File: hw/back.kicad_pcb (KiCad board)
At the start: 2 copper layers, 110 x 55 mm, 77 parts, among them J1 IDC_02X13, J2 FC681495, J3 N42GK-04, Q1 BSC080N03MS, U1 OSRB38C9BA, U2 MCP1826S, U3 MCP1826S, U4 BQ24192, U5 LTC1871, U6 LTC2941CMS8E

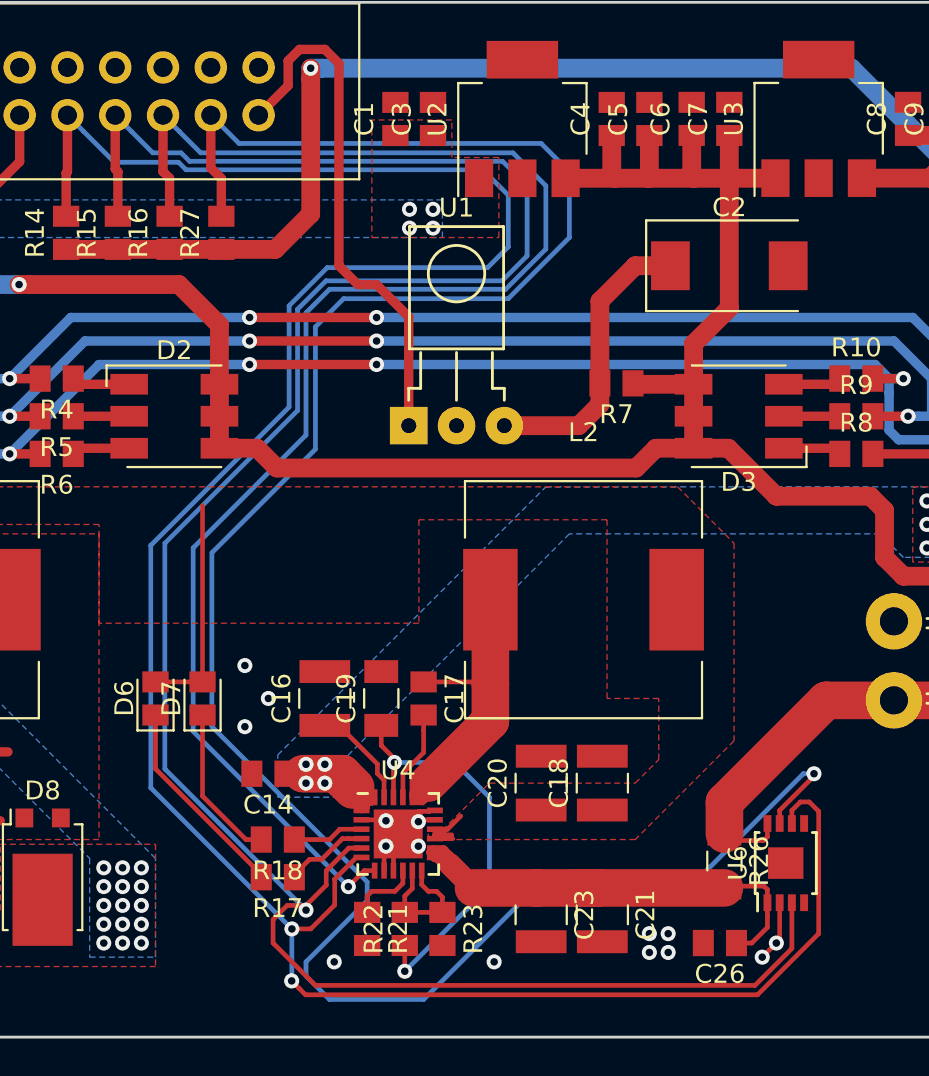
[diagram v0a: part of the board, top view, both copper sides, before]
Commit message: updated pcb
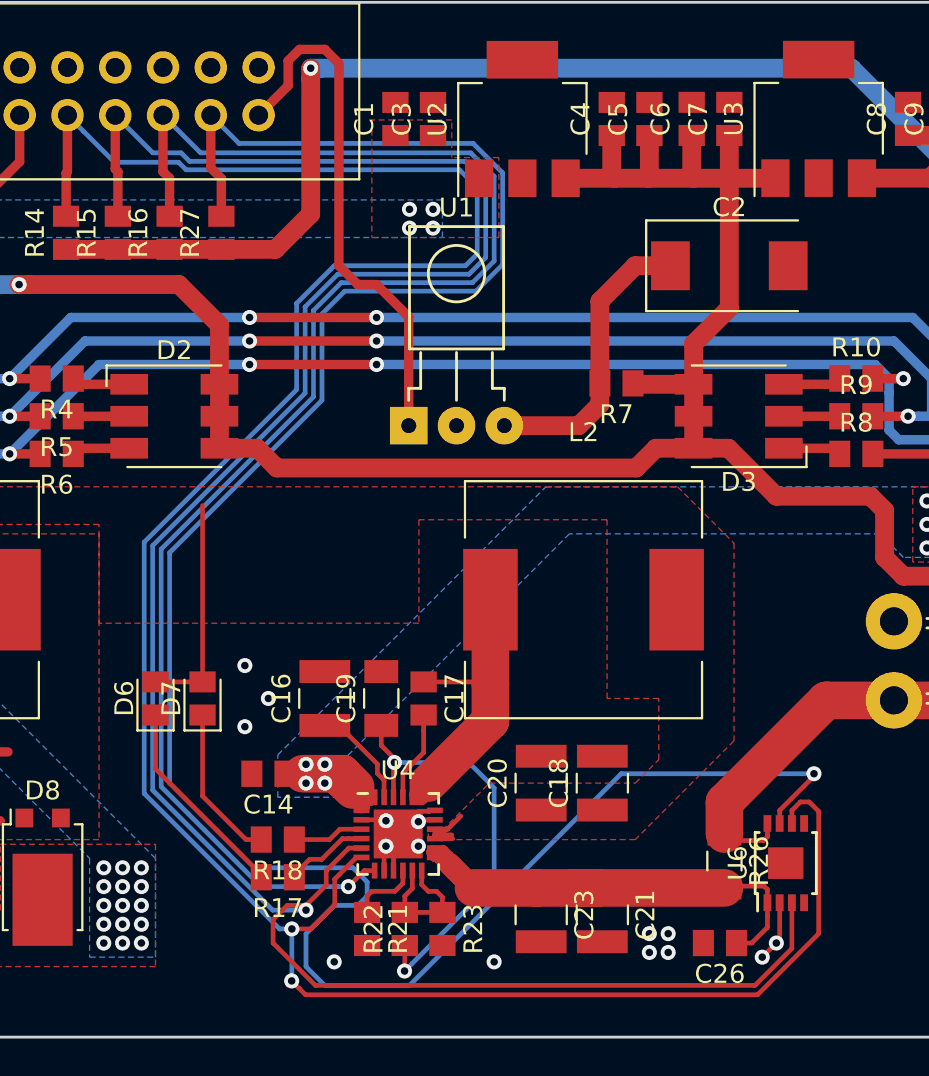
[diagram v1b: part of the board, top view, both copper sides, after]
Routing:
- net /SCL: track 123.9 -> 121.1 mm
- net /SDA: track 133.1 -> 130.8 mm
- net /~AL: track 122.3 -> 121.0 mm
- net /~INT: track 83.1 -> 82.2 mm
- net Net-(C19-Pad1): track 22.7 -> 23.3 mm
